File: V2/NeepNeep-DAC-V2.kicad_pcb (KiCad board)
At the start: 2 copper layers, 24 x 24 mm, 16 parts, among them J1 Conn_02x03_Odd_Even, Q1 MMBT3904, U2 W25Q32JVSS, U3 ATtiny85-20SU

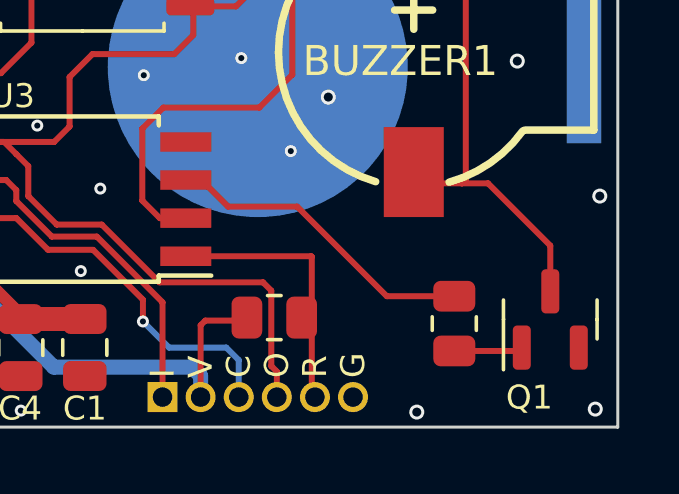
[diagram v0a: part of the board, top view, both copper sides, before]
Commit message: Commit: A	V2/NeepNeep-DAC-V2-backups/NeepNeep-DAC-V2-2026-02-09_174934.zip A	V2/NeepNeep-DAC-V2-backups/NeepNeep-DAC-V2-2026-02-10_125359.zip A	V2/NeepNeep-DAC-V2-backups/NeepNeep-DAC-V2-2026-02-10_130055.zip M	V2/NeepNeep-DAC-V2.kicad_pcb M	V2/NeepNeep-DAC-V2.kicad_prl M	V2/NeepNeep-DAC-V2.kicad_sch A	V2/Thumbs.db
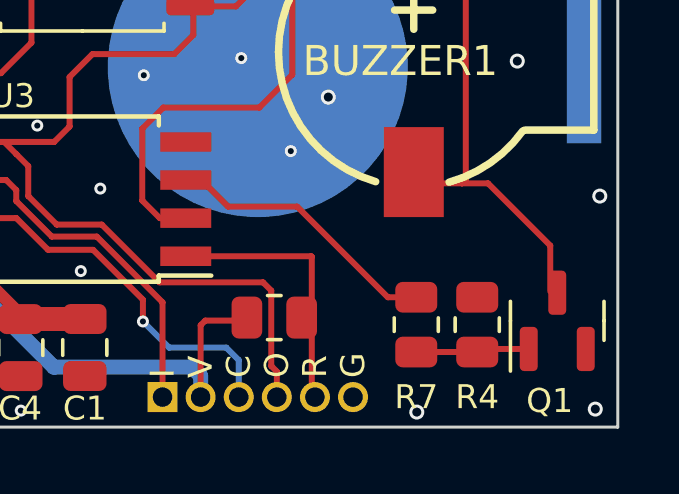
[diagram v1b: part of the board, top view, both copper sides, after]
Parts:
- added R4: 100k, Resistor_SMD:R_0805_2012Metric, F.Cu at (107.3, 108.6)
- Q1: value MMBT3904 -> BSS138
- moved R7 1.27 mm to (105.3, 108.6)
- moved Q1 0.24 mm to (110.0, 108.5)
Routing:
- net Net-(Q1-G): track 2.30 -> 3.79 mm
- net PB4: track 10.6 -> 9.30 mm
